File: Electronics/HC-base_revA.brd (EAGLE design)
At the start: 65.2 x 29.3 mm, 35 parts, among them T2 BSS138, T3 BSS138, T4 BSS138, T5 BSS138, U2 NRF24L01, U3 OLED128X64

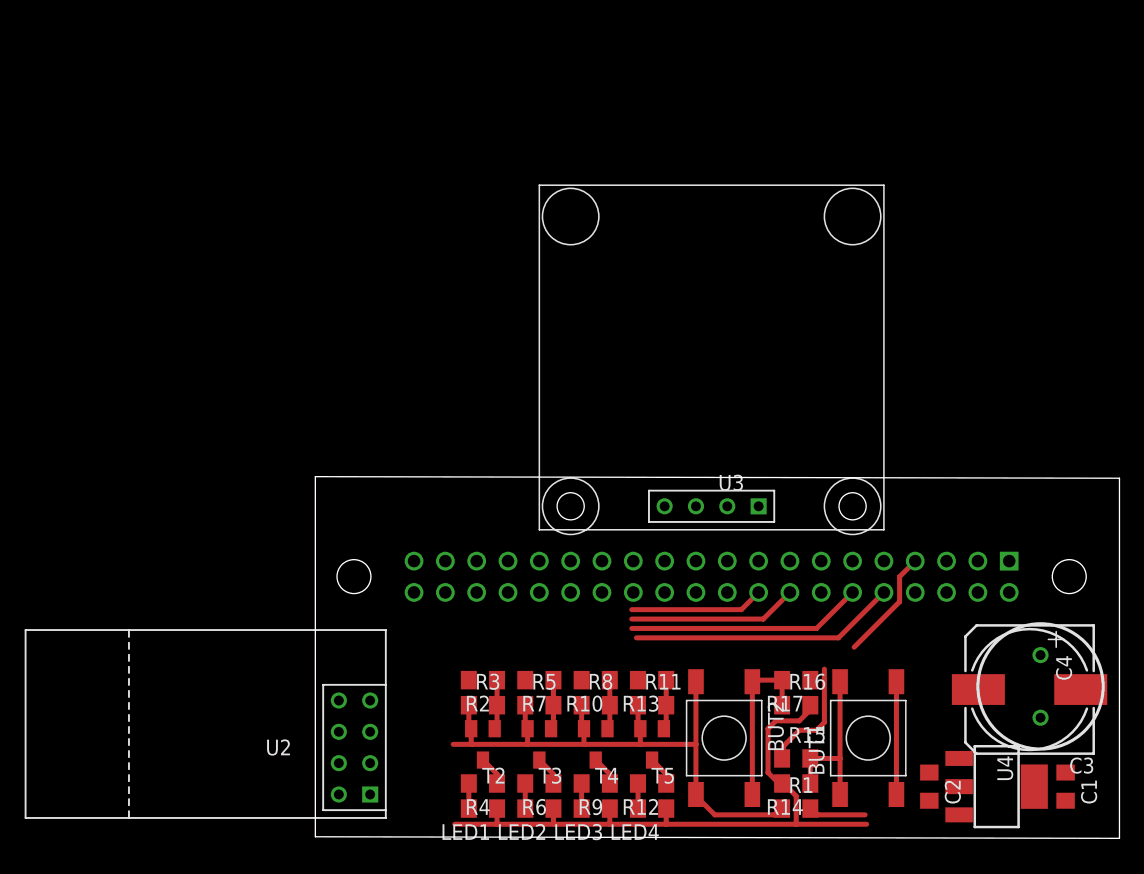
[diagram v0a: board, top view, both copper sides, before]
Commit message: modified: diagram and pcb
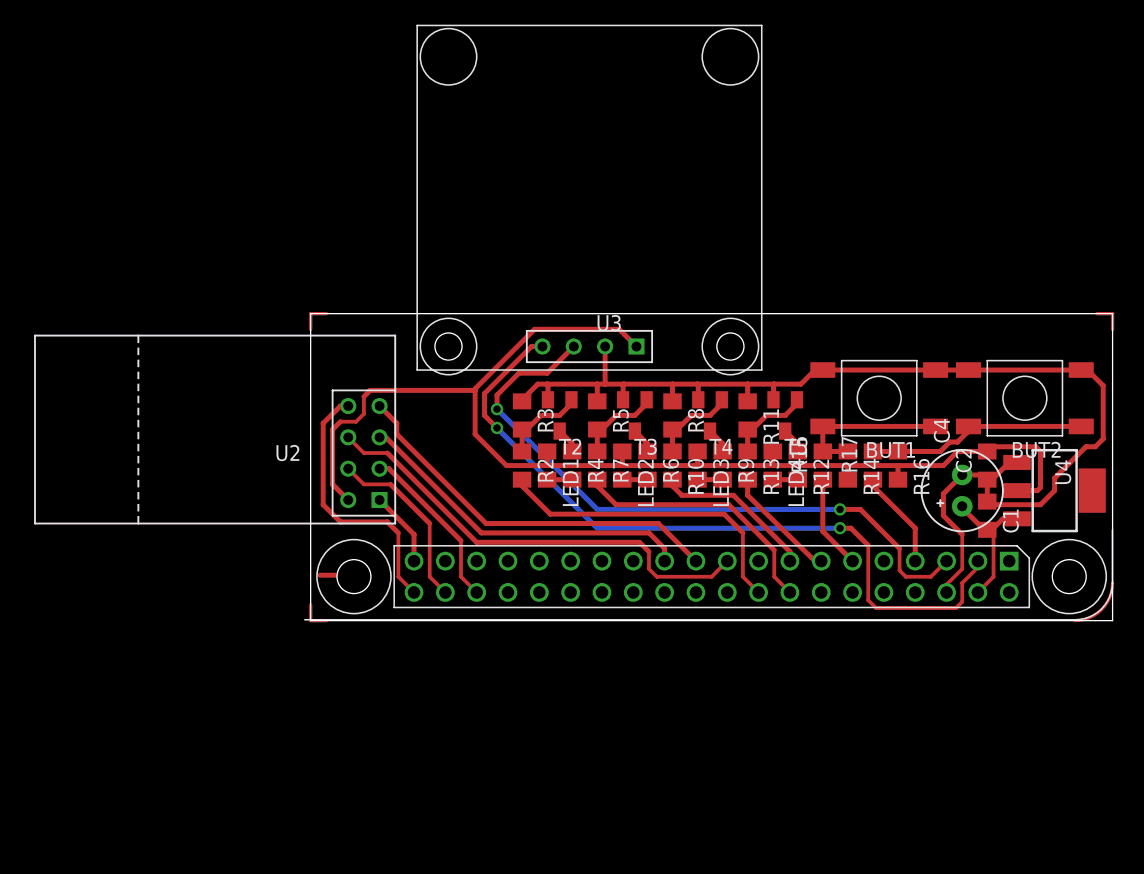
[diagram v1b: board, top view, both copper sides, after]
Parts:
- removed C3: (no value), rcl:153CLV-1012
- removed R1: 0R\, 1_domaci:R0805
- added U$1, U$2, U$3: CORNER, 1_domaci:CORNER
- C4: device 1_domaci:ELYT-10MM -> 1_domaci:ELYT-6MM5
- moved BUT2 36.8 mm to (64.0, 41.1), turned to 180 degrees
- moved LED4 29.5 mm to (43.6, 35.7), turned to 270 degrees
- moved LED3 29.0 mm to (37.5, 35.7), turned to 270 degrees
- moved T5 28.8 mm to (44.6, 39.8)
- moved LED2 28.6 mm to (31.4, 35.7), turned to 270 degrees
- moved R12 28.4 mm to (45.6, 35.7), turned to 270 degrees
- moved LED1 28.3 mm to (25.3, 35.7), turned to 270 degrees
- moved T4 28.2 mm to (38.5, 39.8)
- moved T3 27.8 mm to (32.4, 39.8)
- moved R9 27.8 mm to (39.5, 35.7), turned to 270 degrees
- moved BUT1 27.6 mm to (52.2, 41.1), turned to 180 degrees
- moved T2 27.4 mm to (26.3, 39.8)
- moved R6 27.2 mm to (33.4, 35.7), turned to 270 degrees
- moved R4 26.8 mm to (27.3, 35.7), turned to 270 degrees
- moved C2 26.5 mm to (61.0, 35.7), turned to 90 degrees
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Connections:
- new net N$21: U1.P$39, U2.1
- net +5V: now also C4.+; no longer C4.P
- net BUT1: now also U1.P$11; no longer U1.P$8
- net GND: now also C4.-; no longer C4.N, R1.1, R1.2, U1.P$34, U2.1
- net LED3: now also U1.P$15; no longer U1.P$12
- net LED4: now also U1.P$13; no longer U1.P$10
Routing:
- net N$8: track 0.00 -> 59.9 mm, vias 0 -> 2
- net N$9: track 0.00 -> 52.6 mm, vias 0 -> 2
- net +3V3: track 51.9 -> 98.8 mm
- net N$3: track 0.00 -> 36.8 mm
- net GND: track 63.6 -> 96.1 mm
- net N$4: track 0.00 -> 31.4 mm
- net N$2: track 0.00 -> 27.9 mm
- net N$7: track 0.00 -> 21.6 mm
- net N$5: track 0.00 -> 14.6 mm
- net LED1: track 10.9 -> 25.3 mm
- net N$6: track 0.00 -> 13.7 mm
- net LED4: track 21.6 -> 9.41 mm
- net +5V: track 0.00 -> 11.5 mm
- net LED2: track 13.7 -> 21.0 mm
- net LED3: track 19.1 -> 13.0 mm
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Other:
- board size 65.2 x 29.3 mm -> 65 x 24.9 mm
